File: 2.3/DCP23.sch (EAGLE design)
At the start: 14 parts, among them CON1 USB-1, IC1 STM32F103CBT7, IC2 AP2127-3.3, Q1 8 MHz

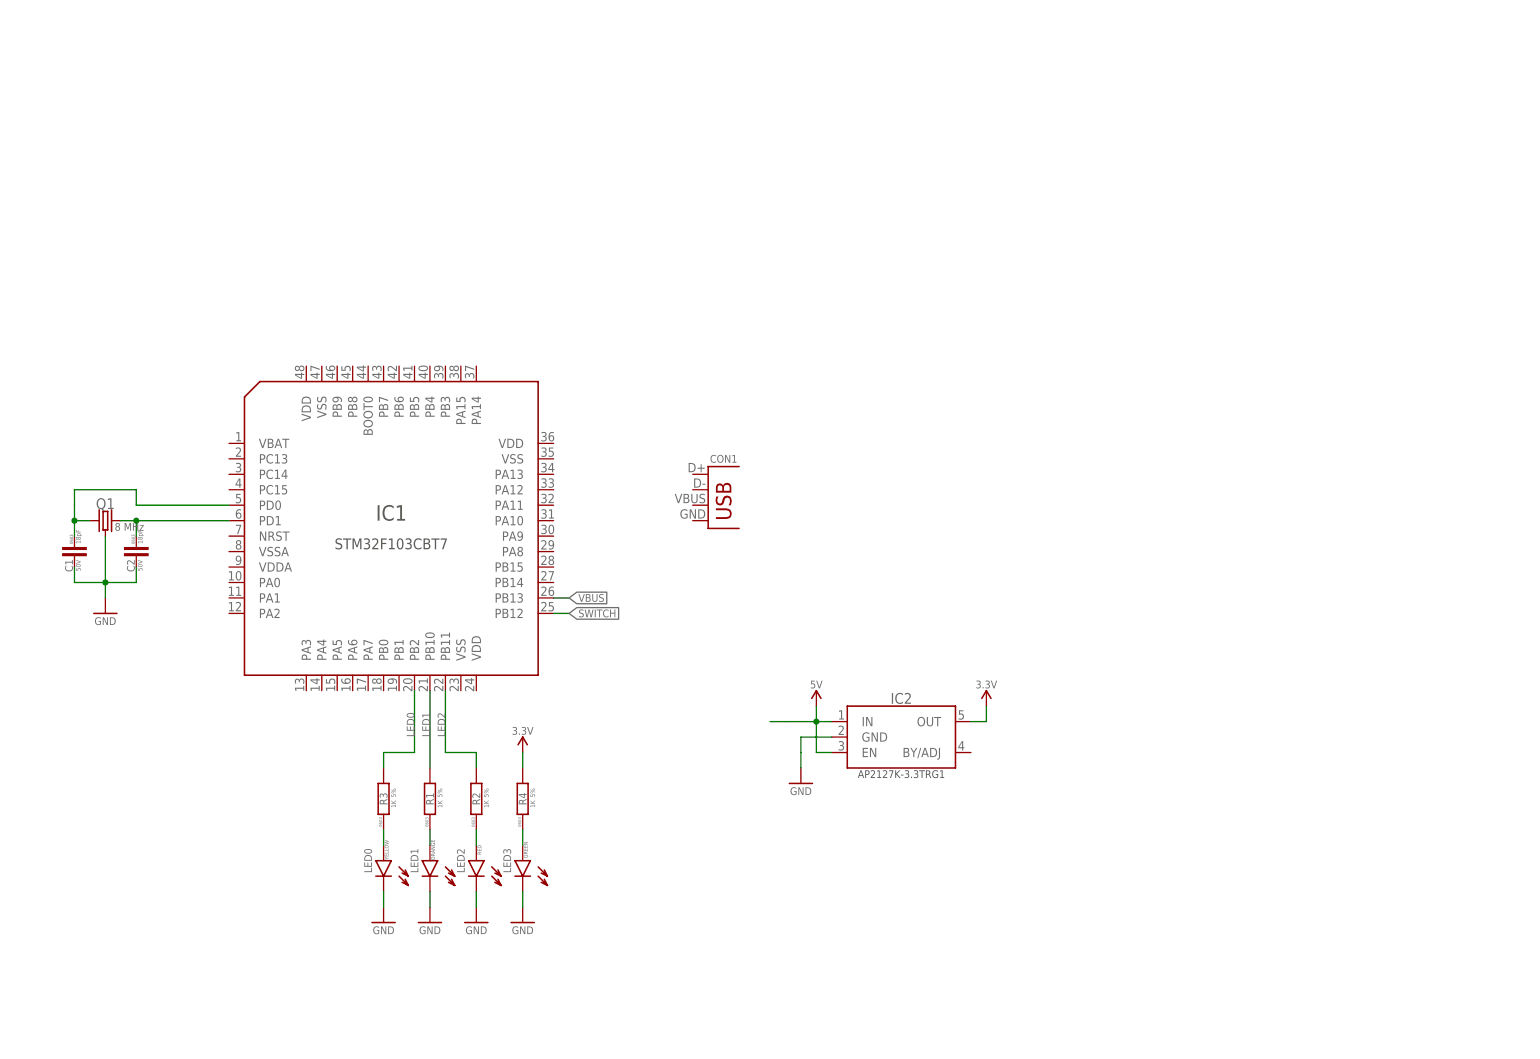
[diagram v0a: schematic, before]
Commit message: 2.3 schematic  completed
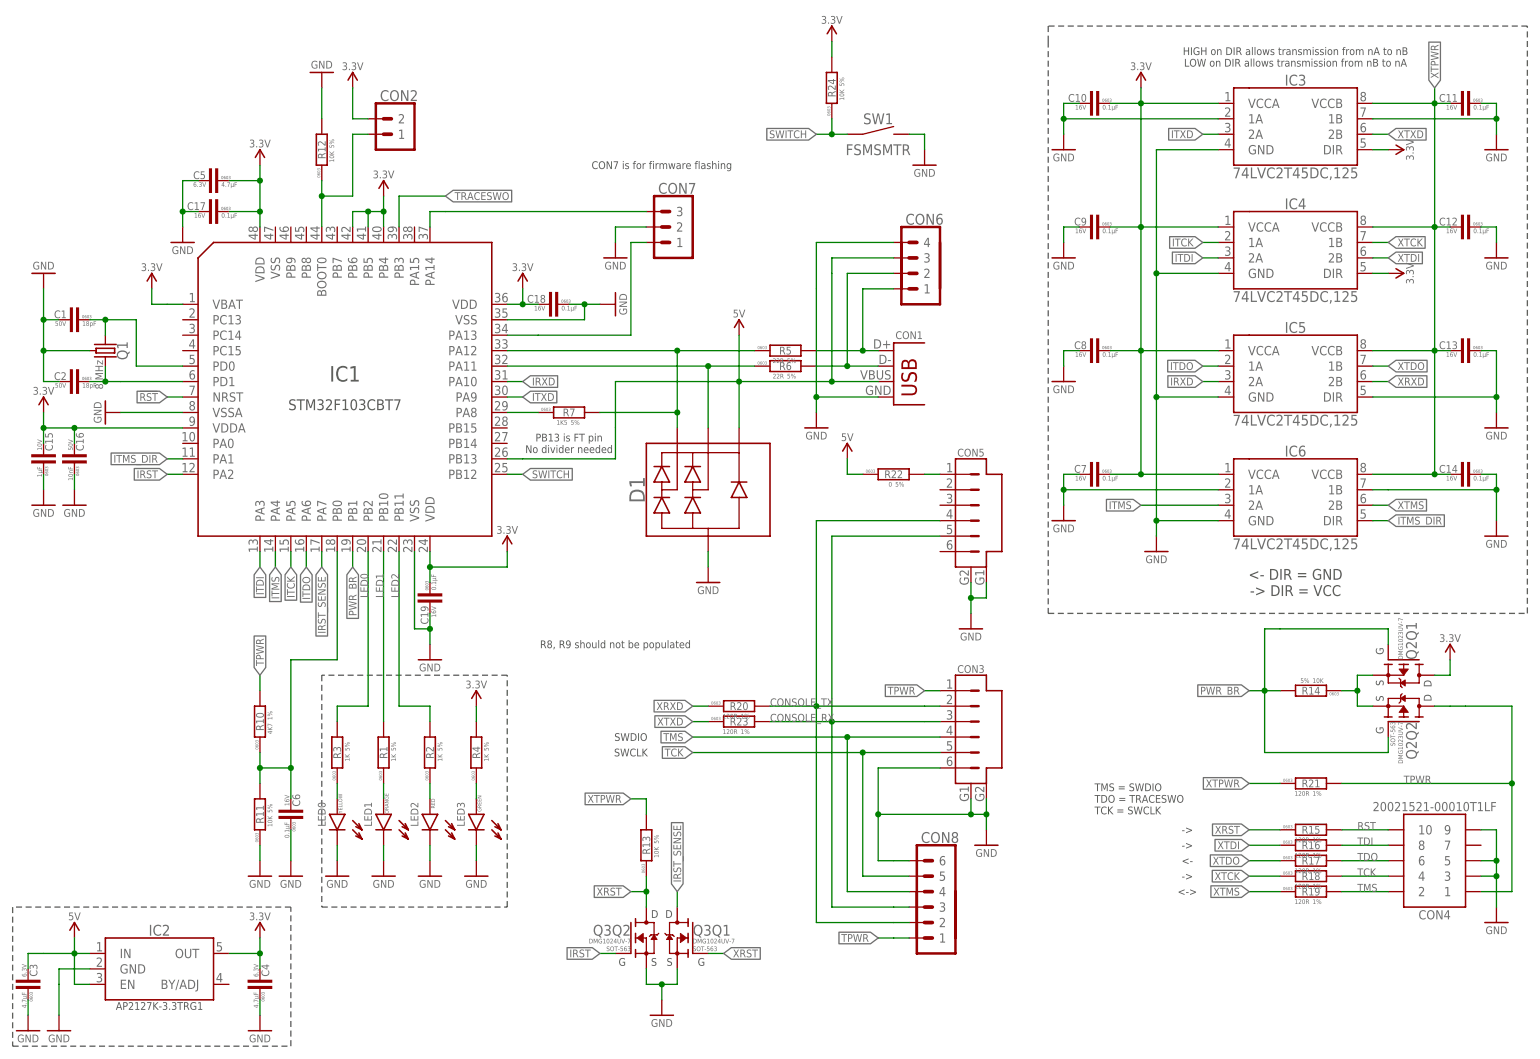
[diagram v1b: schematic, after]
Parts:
- added C10, C11, C12, C13, C14, C17, C18, C19, C6, C7, C8, C9: 0.1µF, C_digikey:0.1µF-16V_10%_X7R-0603
- added C15: 1µF, C_digikey:1µF-10V_10%_X5R-0603
- added C16: 10nF, C_digikey:10NF-50V_10%_X7R-0603
- added C3, C4, C5: 4.7µF, C_digikey:4.7µF-6.3V_10%_X5R-0603
- added CON2: PINHEAD_1X02-2, pinhead:PINHEAD_1X02-2
- added CON3: CON-6P-SM06B, Connectors:CON-6P-SM06B
- added CON4: CON-2X5P, Connectors:CON-2X5P
- added CON5: CON-6P-DF13, Connectors:CON-6P-DF13
- added CON6: PINHEAD_1X04-2.54, pinhead:PINHEAD_1X04-2.54
- added CON7: PINHEAD_1X03-2.54, pinhead:PINHEAD_1X03-2.54
- added CON8: PINHEAD_1X06-2.54, pinhead:PINHEAD_1X06-2.54
- added D1: PRTR5V0U2X, TVS_diodes:PRTR5V0U2X
- added IC3, IC4, IC5, IC6: 74LVC2T45, misc:74LVC2T45
- added Q2: DMG1023UV-7, mosfet:DMG1023UV-7
- added Q3: DMG1024UV-7, mosfet:DMG1024UV-7
- added R10: 4K7, R_digikey:4K7-1%-0603
- added R11, R12, R13, R14, R24: 10K, R_digikey:10K-5%-0603
- added R15, R16, R17, R18, R19, R20, R21, R23: 120R, R_digikey:120R-1%-0603
- added R22: 0, R_digikey:0R-5%-0603
- added R5, R6: 22R, rc:R-5%-0603
- added R7: 1K5, rc:R-5%-0603
- added SW1: TACT_SWITCH-FSMSM, misc:TACT_SWITCH-FSMSM
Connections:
- removed net VBUS: IC1.PB13
- new net !RST: IC1.NRST
- new net CONSOLE_RX: CON3.3, CON5.5, CON8.3, R23.2
- new net CONSOLE_TX: CON3.2, CON5.4, CON8.2, R20.2
- new net IRST: IC1.PA2, Q3Q2.G
- new net IRST_SENSE: IC1.PA7, Q3Q1.D
- new net IRXD: IC1.PA10, IC5.2A
- new net ITCK: IC1.PA5, IC4.1A
- new net ITDI: IC1.PA3, IC4.2A
- new net ITDO: IC1.PA6, IC5.1A
- new net ITMS: IC1.PA4, IC6.2A
- new net ITMS_DIR: IC1.PA1, IC6.DIR
- new net ITXD: IC1.PA9, IC3.2A
- new net N$10: CON1.D-, CON6.2, R6.2
- new net N$11: CON1.D+, CON6.1, R5.2
- new net N$12: Q2Q1.S, Q2Q2.S, R14.1
- new net N$13: CON5.1, R22.2
- new net N$15: CON2.1, IC1.BOOT0, R12.1
- new net N$7: IC1.PA8, R7.1
- new net N$8: D1.D2, IC1.PA11, R6.1
- new net N$9: D1.D1, IC1.PA12, R5.1, R7.2
- new net PWR_BR: IC1.PB1, Q2Q1.G, Q2Q2.G, R14.2
- new net RST: CON4.10, R15.2
- new net SWCLK: CON7.3, IC1.PA14
- new net SWDIO: CON7.1, IC1.PA13
- new net TCK: CON3.5, CON4.4, CON8.5, R18.2
- new net TDI: CON4.8, R16.2
- new net TDO: CON4.6, R17.2
- new net TMS: CON3.4, CON4.2, CON8.4, R19.2
- new net TPWR: CON3.1, CON4.1, CON8.1, Q2Q2.D, R10.2, R21.2
- new net TRACESWO: IC1.PB3
- new net VBUS1: C6.2, IC1.PB0, R10.1, R11.2
- new net XRST: Q3Q1.G, Q3Q2.D, R13.1, R15.1
- new net XRXD: IC5.2B, R20.1
- new net XTCK: IC4.1B, R18.1
- new net XTDI: IC4.2B, R16.1
- new net XTDO: IC5.1B, R17.1
- new net XTMS: IC6.2B, R19.1
- new net XTPWR: C11.2, C12.2, C13.2, C14.2, IC3.VCCB, IC4.VCCB, IC5.VCCB, IC6.VCCB, R13.2, R21.1
- new net XTXD: IC3.2B, R23.1
- net GND: now also C10.2, C11.1, C12.1, C13.1, C14.1, C15.1, C16.1, C17.2, C18.1, C19.2, C3.1, C4.1, C5.2, C6.1, C7.2, C8.2, C9.2, CON1.GND, CON3.6, CON3.G1, CON3.G2, CON4.3, CON4.5, CON4.9, CON5.G1, CON5.G2, CON6.4, CON7.2, CON8.6, D1.C, IC1.VSS@1, IC1.VSS@2, IC1.VSSA, IC3.1A, IC3.1B, IC3.GND, IC4.GND, IC5.DIR, IC5.GND, IC6.1A, IC6.1B, IC6.GND, Q3Q1.S, Q3Q2.S, R11.1, R12.2, SW1.2
- net SWITCH: now also R24.1, SW1.1
- net VDD_3V3: now also C10.1, C15.2, C16.2, C17.1, C18.2, C19.1, C4.2, C5.1, C7.1, C8.1, C9.1, CON2.2, IC1.PB4, IC1.PB5, IC1.PB6, IC1.VBAT, IC1.VDD@1, IC1.VDD@2, IC1.VDD@3, IC1.VDDA, IC3.DIR, IC3.VCCA, IC4.DIR, IC4.VCCA, IC5.VCCA, IC6.VCCA, Q2Q1.D, R24.2
- net VDD_5V: now also C3.2, CON1.VBUS, CON6.3, D1.A, IC1.PB13, R22.1
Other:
- note added: "->"
- note added: "<-"
- note added: "<- DIR = GND -> DIR = VCC"
- note added: "<->"
- note added: "CON7 is for firmware flashing"
- note added: "HIGH on DIR allows transmission from nA to nB LOW on DIR allows transmission from nB to nA"
- note added: "PB13 is FT pin No divider needed"
- note added: "R8, R9 should not be populated"
- note added: "SWCLK"
- note added: "SWDIO"
- note added: "TMS = SWDIO TDO = TRACESWO TCK = SWCLK"
- moved on the sheet: C1, C2, CON1, IC1, IC2, LED0, LED1, LED2, LED3, Q1, R1, R2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
